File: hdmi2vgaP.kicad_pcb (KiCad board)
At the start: 2 copper layers, 54.4 x 26.4 mm, 27 parts, among them J1 HDMI, J2 VGA, J3 Composite

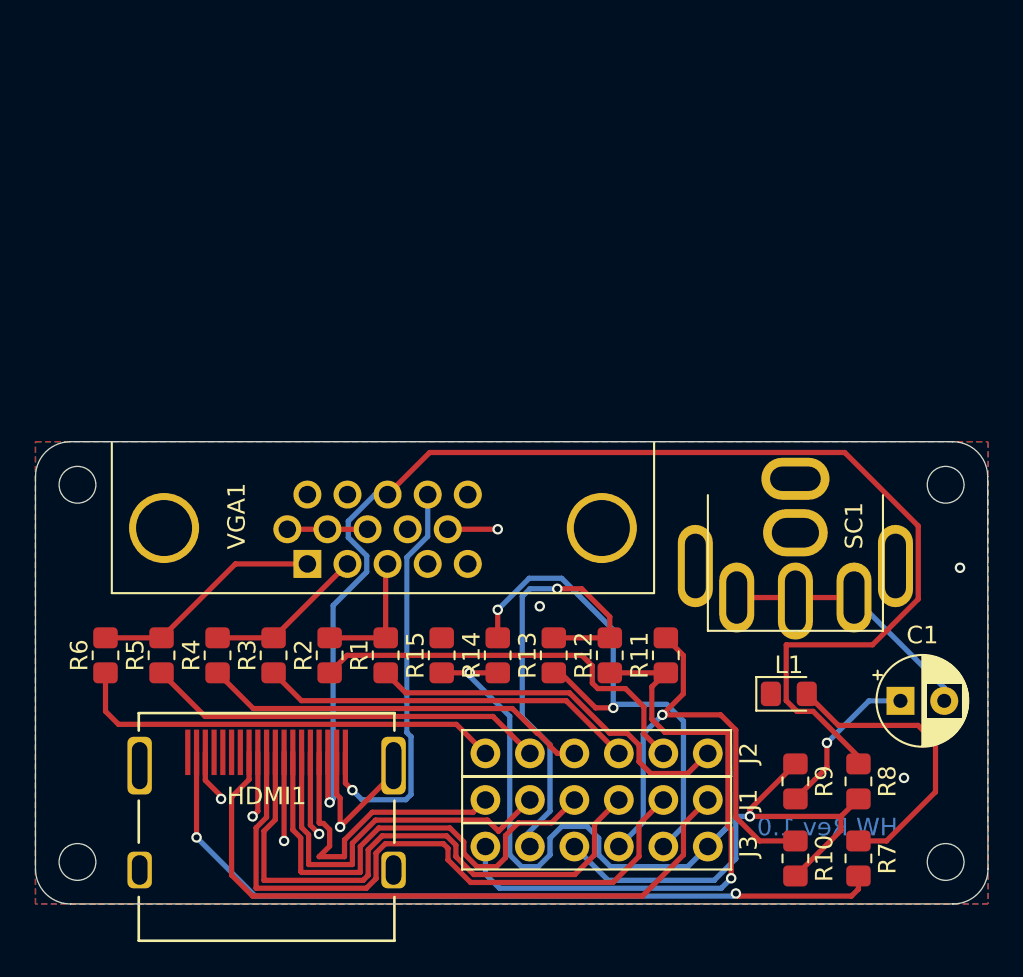
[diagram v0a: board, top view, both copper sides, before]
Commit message: HW Rev 2.0
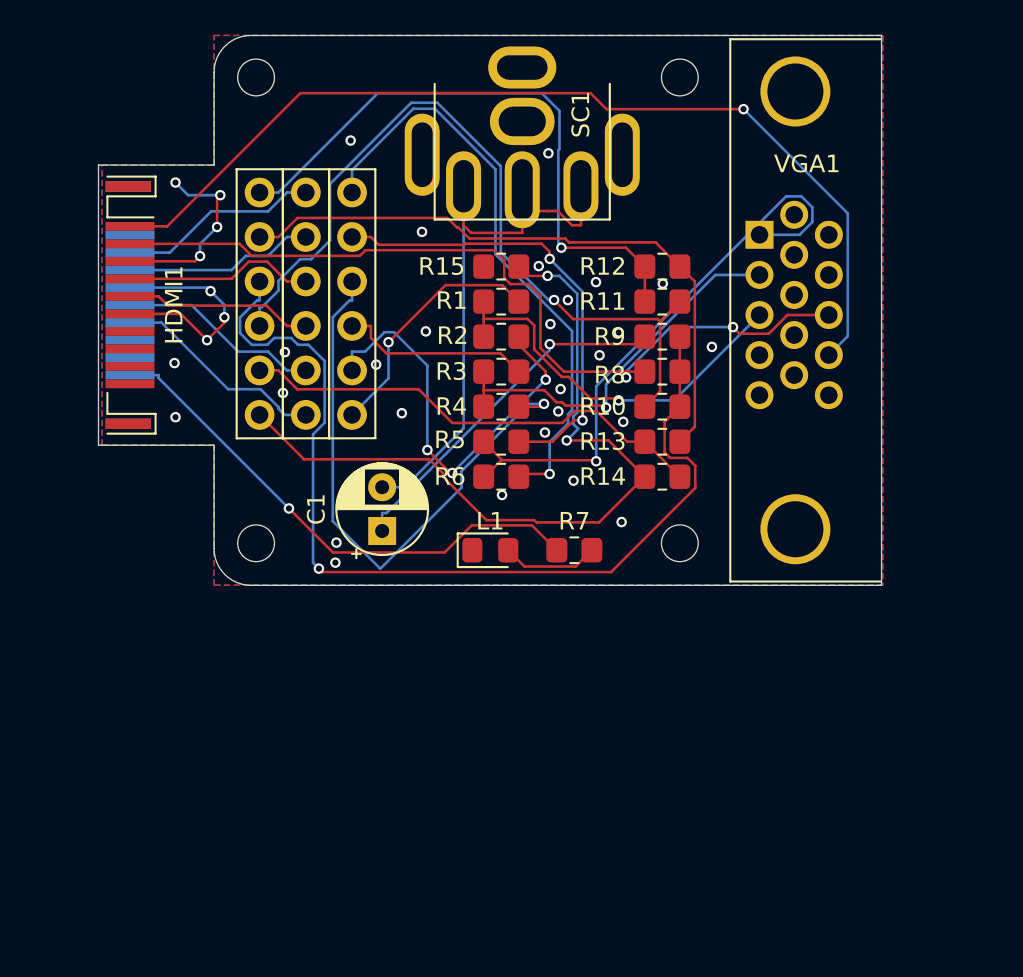
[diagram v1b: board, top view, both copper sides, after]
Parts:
- removed REF** (x4): MountingHole_2.1mm, LIBS:MountingHole_2.1mm
- added H1: MountingHole, MountingHole:MountingHole_2.1mm, F.Cu at (92.6, 23.2)
- added H2: MountingHole, MountingHole:MountingHole_2.1mm, F.Cu at (92.6, 49.8)
- added H3: MountingHole, MountingHole:MountingHole_2.1mm, F.Cu at (68.4, 49.8)
- added H4: MountingHole, MountingHole:MountingHole_2.1mm, F.Cu at (68.4, 23.2)
- HDMI1: footprint LIBS:HDMI -> Connector_Video:HDMI_A_Contact_Technology_HDMI-19APL2_Horizontal
- moved J3 35.5 mm to (68.6, 42.5), turned to 180 degrees
- moved VGA1 31.9 mm to (97.2, 32.2), turned to 90 degrees
- moved J1 31.8 mm to (71.2, 42.5), turned to 180 degrees
- moved C1 31.1 mm to (75.6, 49.1), turned to 90 degrees
- moved SC1 28.2 mm to (83.6, 26.3)
- moved J2 28.0 mm to (73.9, 42.5), turned to 180 degrees
- moved HDMI1 27.4 mm to (61.2, 36.2), turned to -90 degrees
- moved R10 26.9 mm to (91.6, 42.0), turned to 0 degrees
- moved R9 26.5 mm to (91.6, 38.0), turned to 180 degrees
- moved R8 25.9 mm to (91.6, 40.0), turned to 0 degrees
- moved R6 24.8 mm to (82.4, 46.0), turned to 180 degrees
- moved R7 23.9 mm to (86.6, 50.2), turned to 0 degrees
- moved R5 22.9 mm to (82.4, 44.0), turned to 180 degrees
- moved R15 22.5 mm to (82.4, 34.0), turned to 0 degrees
- moved R12 22.4 mm to (91.6, 34.0), turned to 180 degrees
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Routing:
- net /HDMI/D2P: track 23.8 -> 55.5 mm
- net /HDMI/D2N: track 78.0 -> 48.9 mm, vias 1 -> 2
- net /Soft Composite/D0P: track 28.9 -> 55.4 mm
- net /HDMI/CLKN: track 38.4 -> 12.3 mm
- net /HDMI/CLKP: track 37.5 -> 11.6 mm
- net /HDMI/D0N: track 33.8 -> 10.7 mm
- net /VGA/VGA_RH: track 13.3 -> 33.8 mm, vias 0 -> 1
- net /Soft Composite/CVBS: track 14.7 -> 34.0 mm
- net /Soft Composite/D0N: track 27.4 -> 45.9 mm
- net /HDMI/D0P: track 28.2 -> 10.9 mm
- net /HDMI/VBUS: track 45.1 -> 29.9 mm, vias 2 -> 1
- net /VGA/VGA_BH: track 7.47 -> 22.5 mm, vias 0 -> 1
- net /VGA/VGA_GH: track 9.17 -> 22.1 mm, vias 0 -> 1
- net Net-(L1-A): track 16.9 -> 5.55 mm
- net Net-(C1-Pad1): track 9.14 -> 20.4 mm
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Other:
- board size 54.4 x 26.4 mm -> 44.7 x 31.4 mm
- board text added: "HW REV 2.0"
- board text added: "RH1.DEV"
- board text removed: "HW Rev 1.0"
- board text removed: "rh1.dev"
